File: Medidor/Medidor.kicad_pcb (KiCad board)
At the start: 2 copper layers, 93.3 x 43.8 mm, 43 parts, among them J1 TC2030-CTX-TAG_CONECT, SW1 Rotary_Encoder_Switch, SW2 SW_DPST_x2, U1 INA219-INA, U2 Serial, U3 2450AT18D0100, X1 32MHz

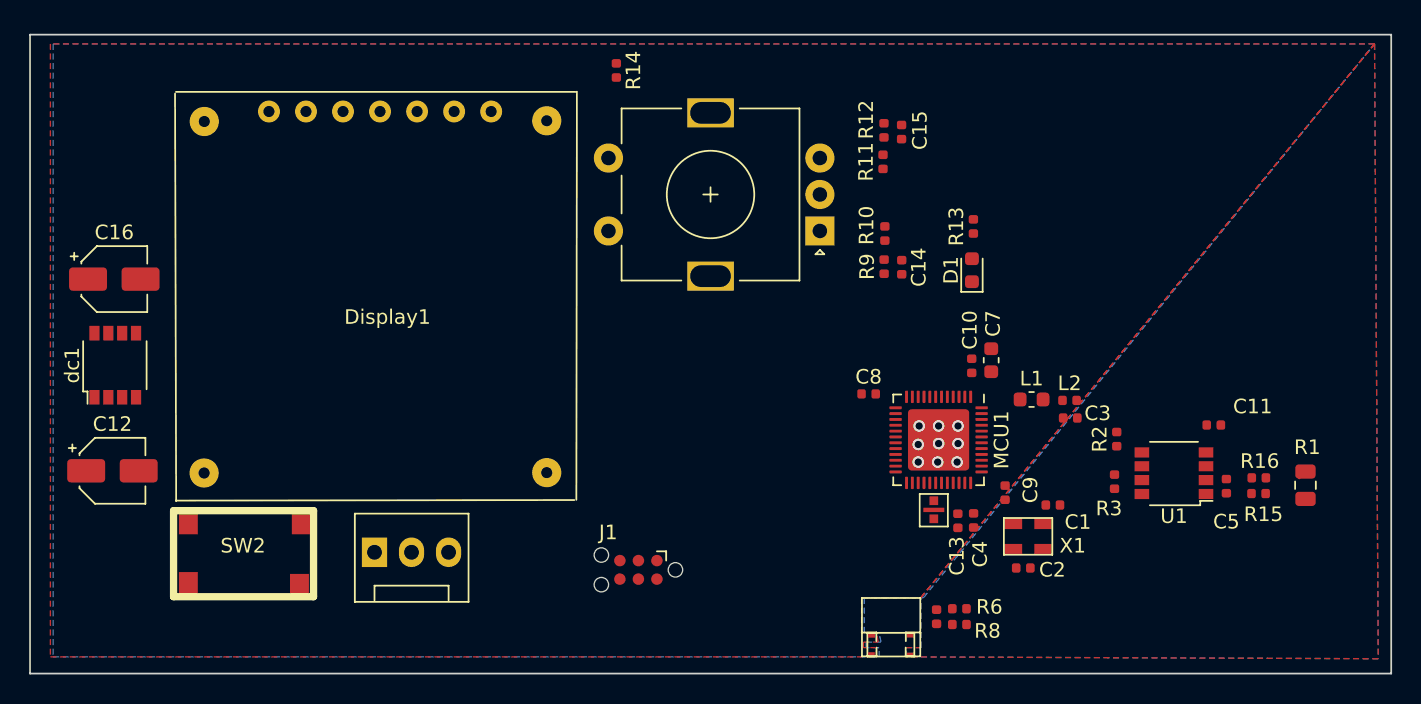
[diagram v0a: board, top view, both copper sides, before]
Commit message: Add files via upload
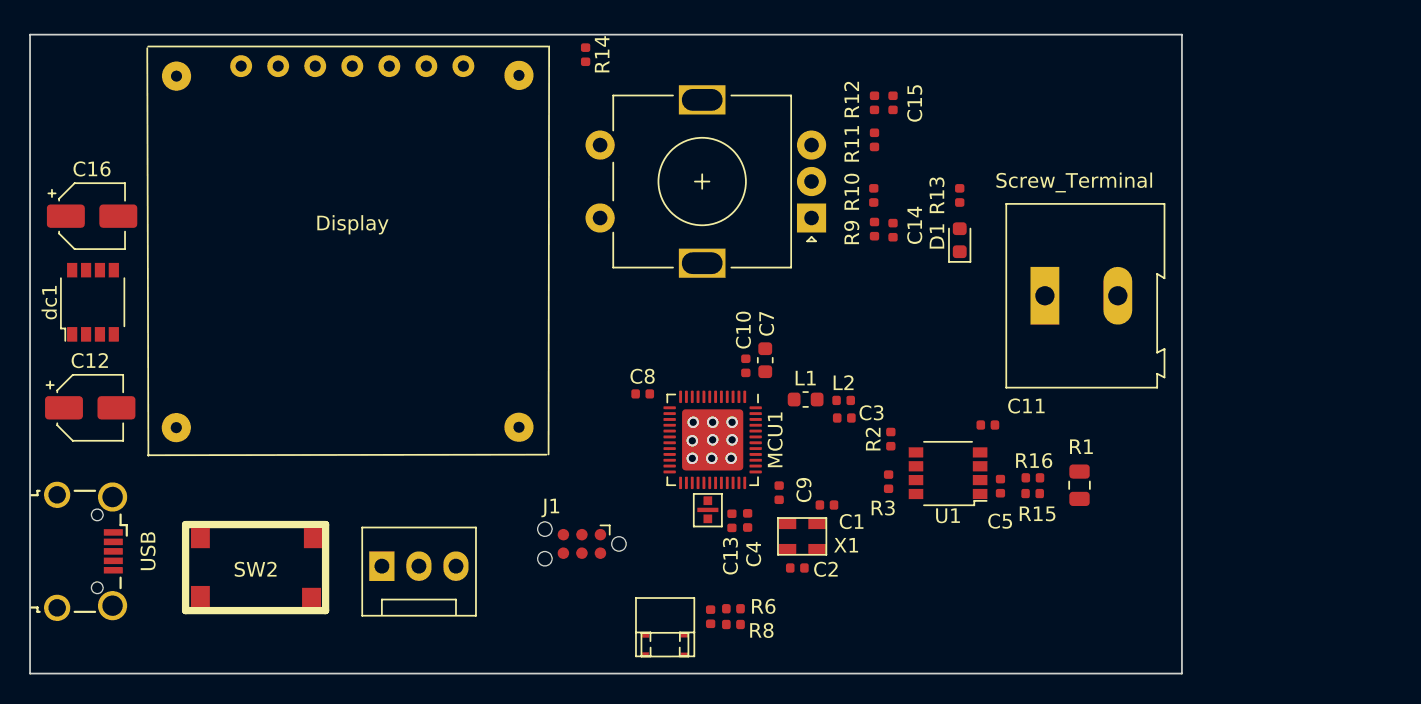
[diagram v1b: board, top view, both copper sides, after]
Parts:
- removed Display1: OLED, Medidor:OLED
- added Display: OLED, Medidor:OLED, F.Cu at (91.9, 103.1)
- added Screw_Terminal: TerminalBlock_Altech_AK300-2_P5.00mm, TerminalBlock:TerminalBlock_Altech_AK300-2_P5.00mm, F.Cu at (139.4, 106.2)
- added USB: USB_Micro-B_Wuerth_629105150521_CircularHoles, Connector_USB:USB_Micro-B_Wuerth_629105150521_CircularHoles, F.Cu at (73.7, 123.7)
- moved C3 15.5 mm to (125.7, 114.6)
- moved MCU1 15.5 mm to (116.7, 116.1)
- moved R7 15.5 mm to (116.5, 128.2)
- moved X1 15.5 mm to (124.5, 121.4)
- moved C11 15.5 mm to (135.5, 115.0)
- moved C13 15.5 mm to (118.0, 121.6)
- moved C2 15.5 mm to (122.5, 124.8)
- moved C4 15.5 mm to (119.1, 121.6)
- moved C5 15.5 mm to (136.4, 119.2)
- moved C7 15.5 mm to (120.3, 110.6)
- moved C8 15.5 mm to (111.9, 112.9)
- moved Fil1 15.5 mm to (116.3, 120.8)
- moved L1 15.5 mm to (123.0, 113.3)
- moved R1 15.5 mm to (141.8, 119.2)
- moved R15 15.5 mm to (138.6, 119.7)
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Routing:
- net Net-(R1-Pad1): track 0.61 -> 0.00 mm
- net Net-(R1-Pad2): track 0.52 -> 0.00 mm
- removed copper zone on B.Cu, net GND
- removed copper zone on F.Cu, net GND
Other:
- board size 93.3 x 43.8 mm -> 79 x 43.8 mm
